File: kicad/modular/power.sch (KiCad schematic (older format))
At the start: 23 parts, among them J1 CONN_PWR, J2 HEADER, U1 LM317, U2 LM337

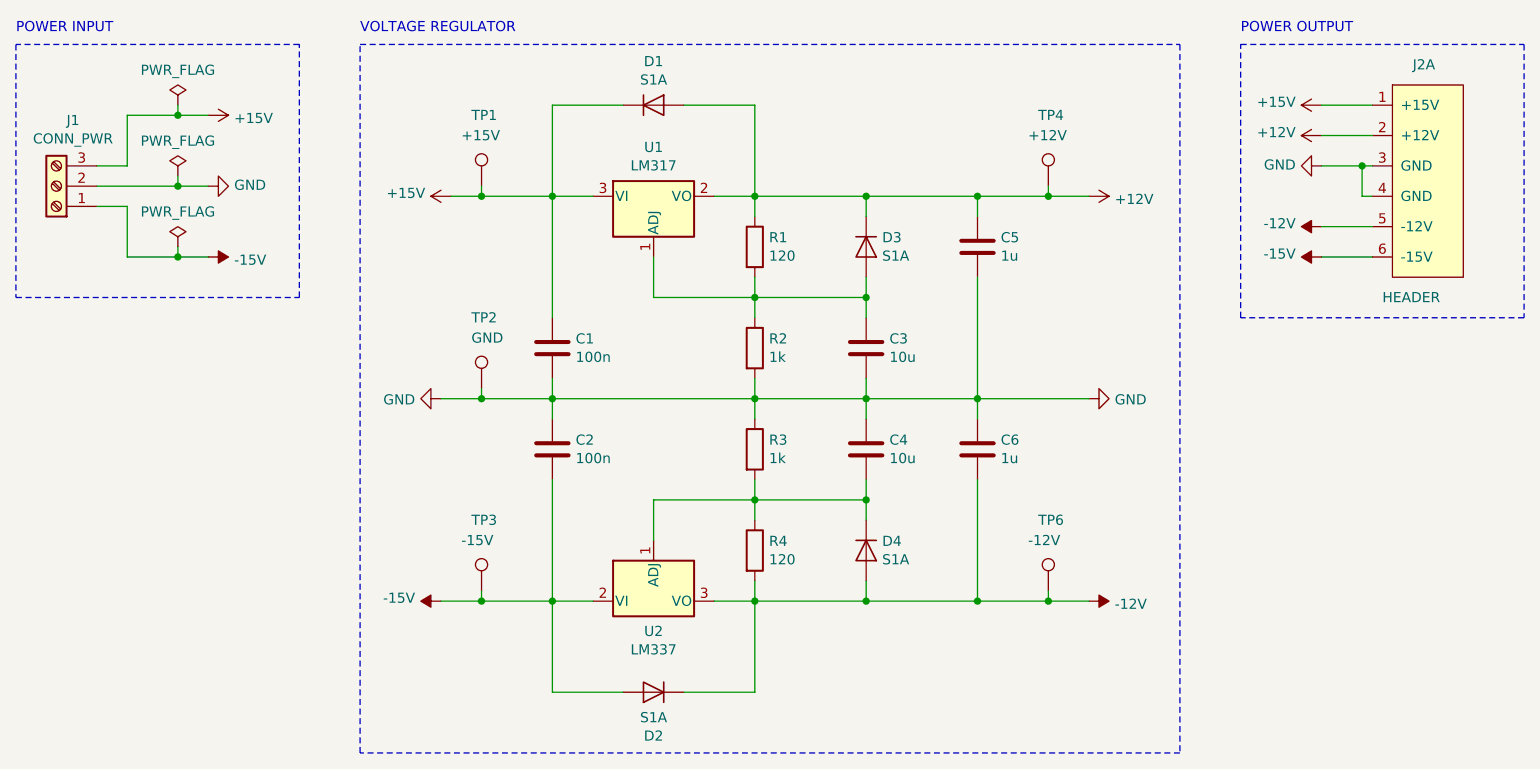
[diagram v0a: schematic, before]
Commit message: started redesign of pcb
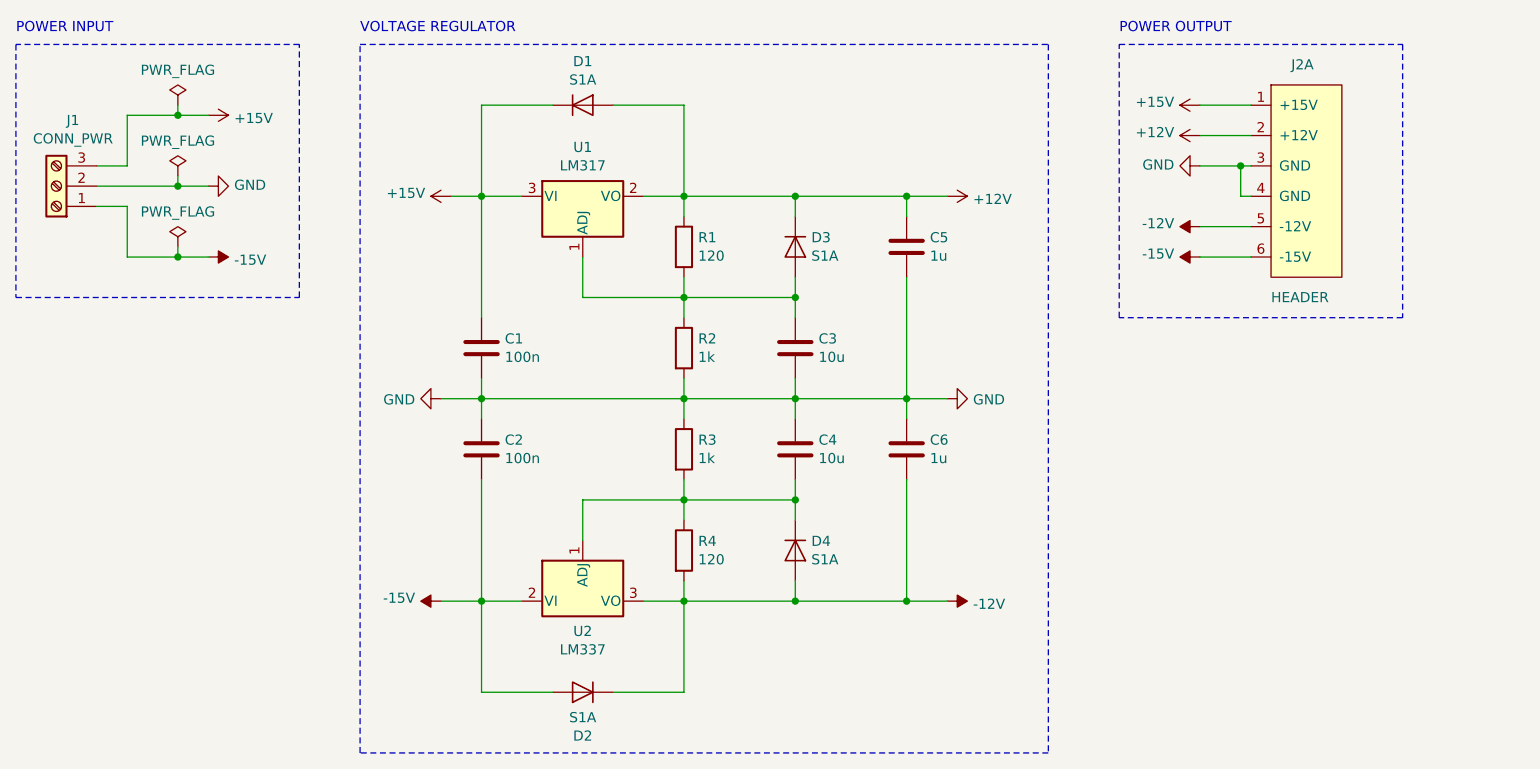
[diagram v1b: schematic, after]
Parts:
- removed TP1: +15V, TestPoint:TestPoint_THTPad_D1.0mm_Drill0.5mm, symbol Connector:TestPoint
- removed TP2: GND, TestPoint:TestPoint_THTPad_D1.0mm_Drill0.5mm, symbol Connector:TestPoint
- removed TP3: -15V, TestPoint:TestPoint_THTPad_D1.0mm_Drill0.5mm, symbol Connector:TestPoint
- removed TP4: +12V, TestPoint:TestPoint_THTPad_D1.0mm_Drill0.5mm, symbol Connector:TestPoint
- removed TP6: -12V, TestPoint:TestPoint_THTPad_D1.0mm_Drill0.5mm, symbol Connector:TestPoint
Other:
- moved on the sheet: C1, C2, C3, C4, C5, C6, D1, D2, D3, D4, J2A, R1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
